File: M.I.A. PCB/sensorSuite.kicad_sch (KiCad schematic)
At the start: 21 parts, among them J2 Conn_Coaxial, U3 MMC5983MA, U4 ICM-45686, U5 MS5611-01BA, U6 TMP117xxDRV, U7 MAX-M10S, U8 KX134-1211

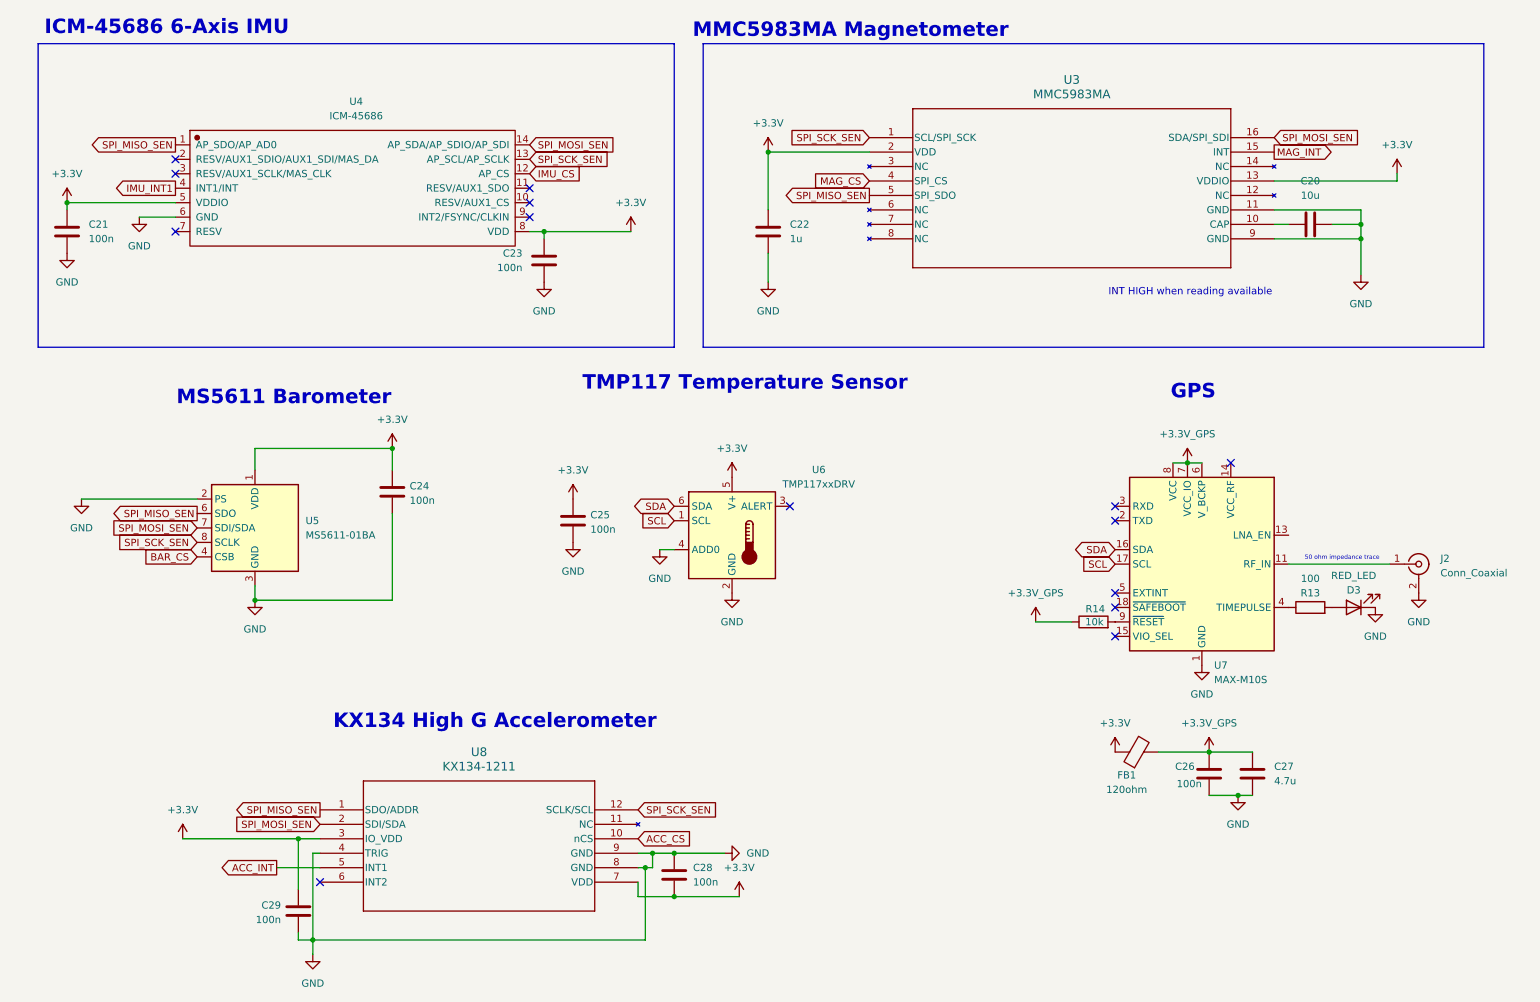
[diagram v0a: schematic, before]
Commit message: More Small Updates/Improvements
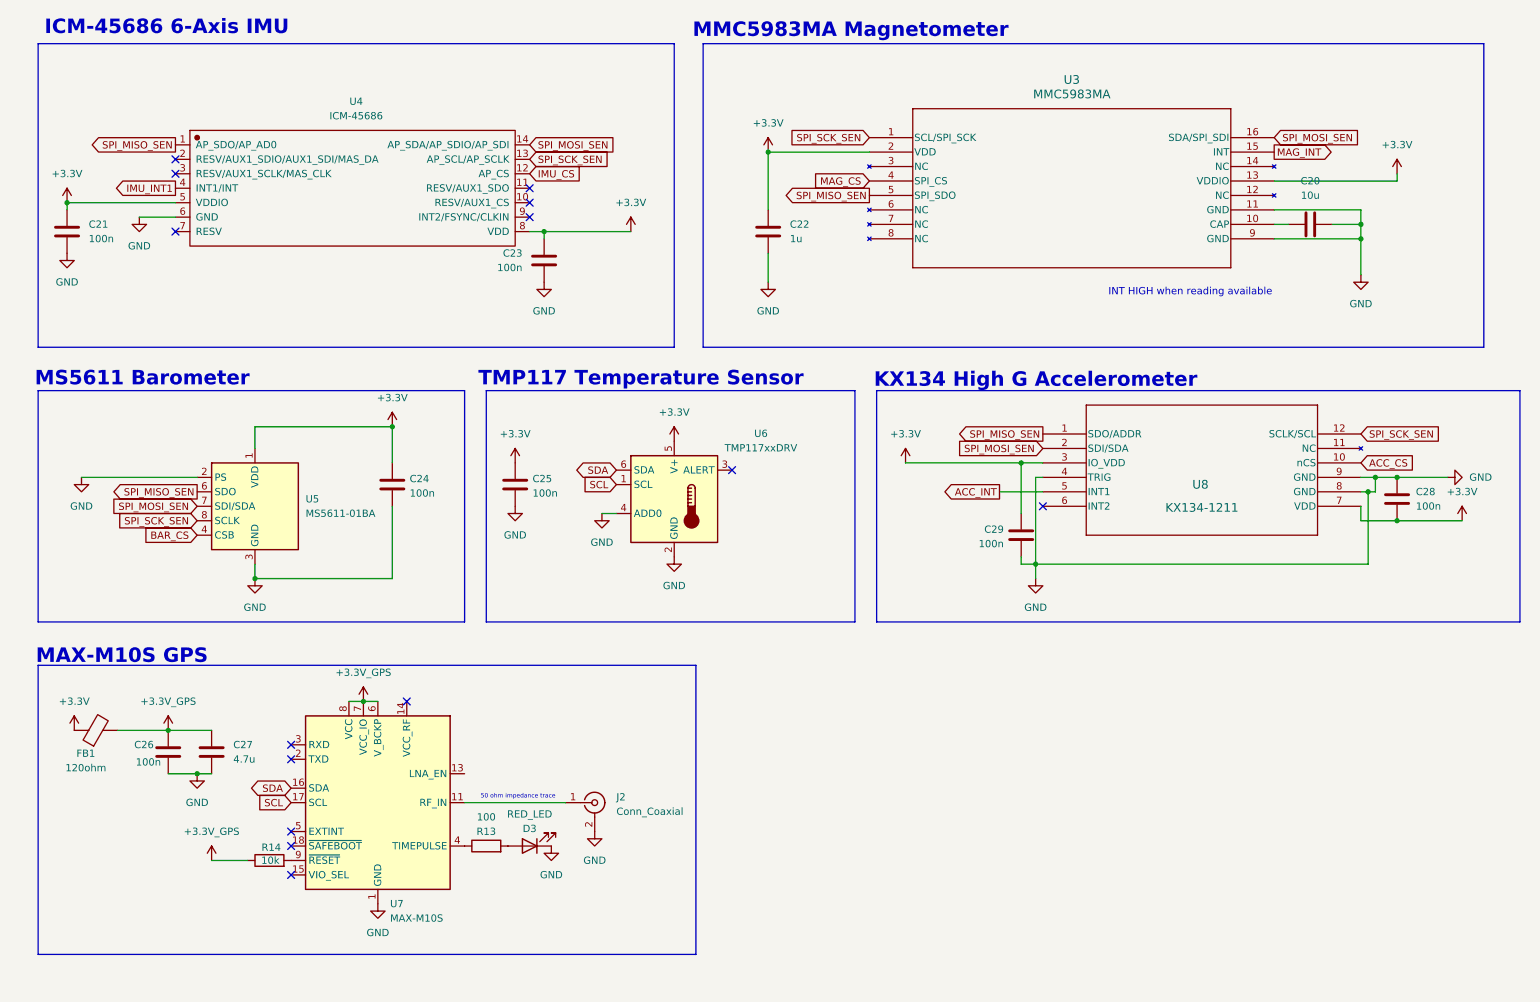
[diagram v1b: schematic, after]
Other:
- note added: "MAX-M10S GPS"
- note removed: "GPS"
- moved on the sheet: C24, C25, C26, C27, C28, C29, D3, FB1, J2, R13, R14, U5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
